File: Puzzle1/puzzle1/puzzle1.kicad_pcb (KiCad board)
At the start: 2 copper layers, 125 x 100 mm, 28 parts, among them J1 Conn_01x04_Pin, J10 Conn_01x09_Socket, J11 Conn_01x04_Socket, J12 Conn_01x04_Socket, J13 Conn_01x04_Socket, J14 Conn_01x04_Socket, J2 Conn_01x09_Socket, J3 Conn_01x09_Socket, J4 Conn_01x09_Socket, J5 Conn_01x09_Socket, J6 Conn_01x09_Socket, J7 Conn_01x09_Socket, J8 Conn_01x09_Socket, J9 Conn_01x09_Socket, U1 PCA9555D, U2 PCA9555D, U3 PCA9555D, U4 PCA9555D, U5 PCA9555D, U6 PCA9555D

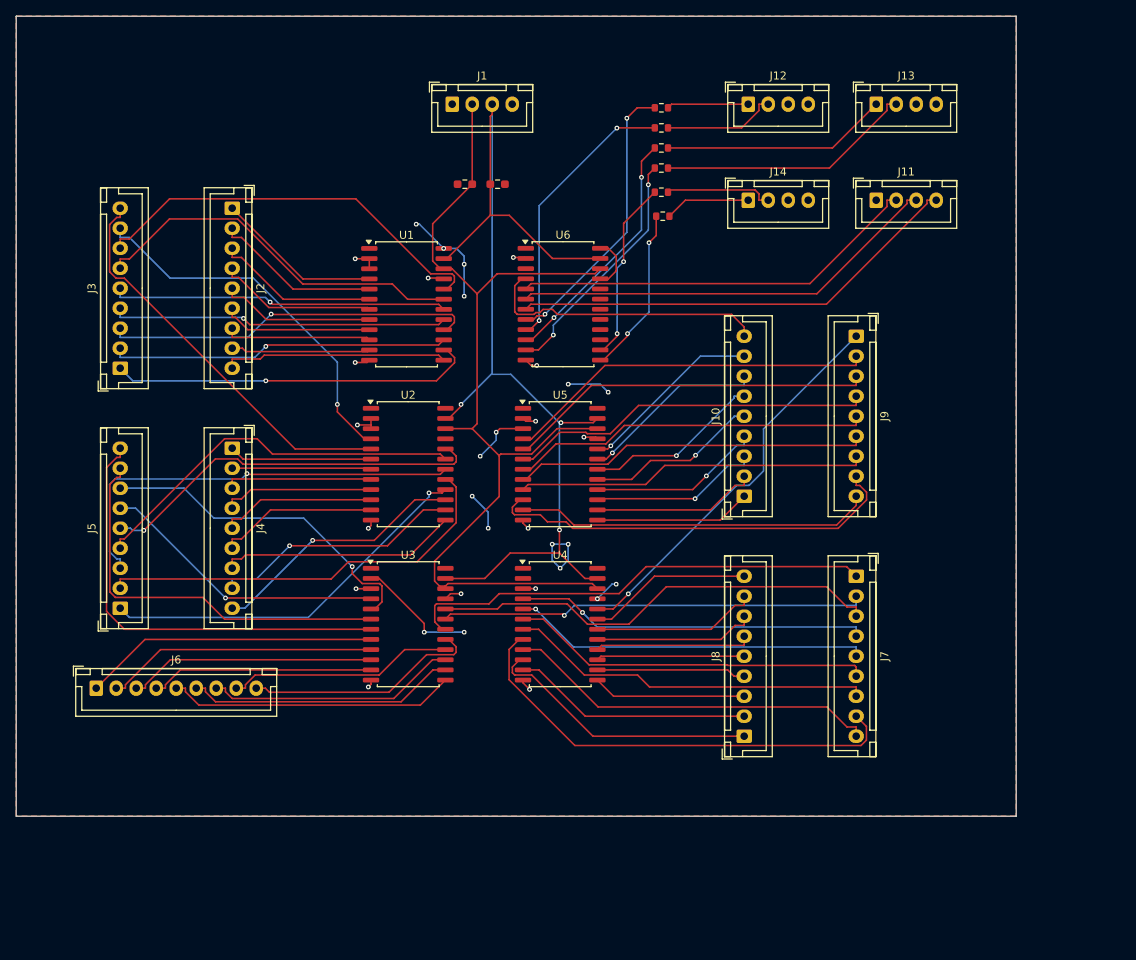
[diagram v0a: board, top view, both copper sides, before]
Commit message: update after review
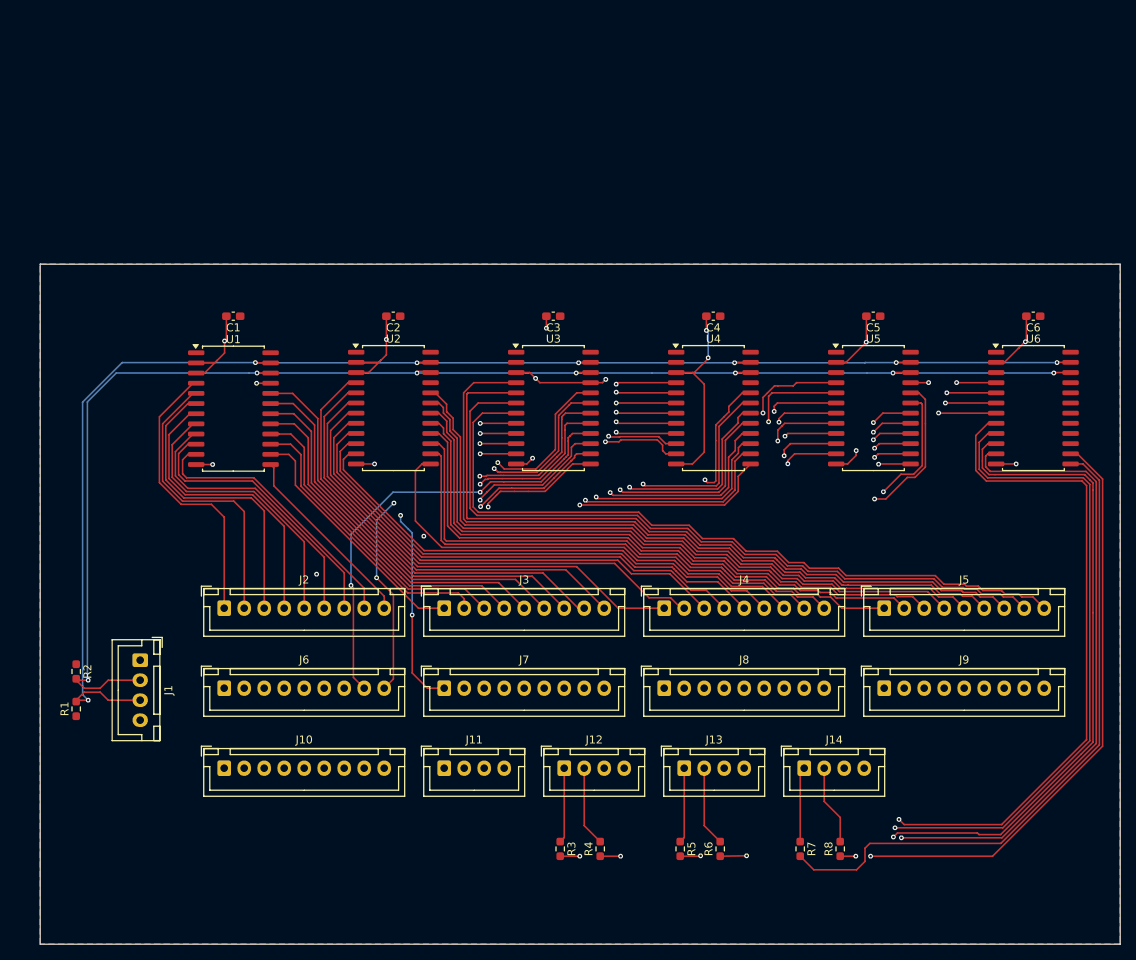
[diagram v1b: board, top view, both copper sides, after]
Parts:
- added C1: 100n, Capacitor_SMD:C_0603_1608Metric_Pad1.08x0.95mm_HandSolder, F.Cu at (49.1, 56.5)
- added C2: 100n, Capacitor_SMD:C_0603_1608Metric_Pad1.08x0.95mm_HandSolder, F.Cu at (69.1, 56.5)
- added C3: 100n, Capacitor_SMD:C_0603_1608Metric_Pad1.08x0.95mm_HandSolder, F.Cu at (89.1, 56.5)
- added C4: 100n, Capacitor_SMD:C_0603_1608Metric_Pad1.08x0.95mm_HandSolder, F.Cu at (109.1, 56.5)
- added C5: 100n, Capacitor_SMD:C_0603_1608Metric_Pad1.08x0.95mm_HandSolder, F.Cu at (129.1, 56.5)
- added C6: 100n, Capacitor_SMD:C_0603_1608Metric_Pad1.08x0.95mm_HandSolder, F.Cu at (149.1, 56.5)
- J10, J2, J3, J4, J5, J6, J7, J8, J9: value Conn_01x09_Socket -> Conn_01x09_Pin
- J11, J12, J13, J14: value Conn_01x04_Socket -> Conn_01x04_Pin
- R3, R4, R5, R6, R7, R8: footprint Resistor_SMD:R_0603_1608Metric -> Resistor_SMD:R_0603_1608Metric_Pad0.98x0.95mm_HandSolder
- moved J5 95.5 mm to (130.5, 93.0), turned to 0 degrees
- moved R3 93.5 mm to (90.0, 123.1), turned to -90 degrees
- moved R4 90.5 mm to (95.0, 123.1), turned to 90 degrees
- moved J11 89.2 mm to (75.5, 113.0)
- moved R5 87.6 mm to (105.0, 123.1), turned to -90 degrees
- moved J13 86.4 mm to (105.5, 113.0)
- moved J12 86.1 mm to (90.5, 113.0)
- moved R6 85.4 mm to (110.0, 123.1), turned to 90 degrees
- moved R8 85.1 mm to (125.0, 123.1), turned to 90 degrees
- moved R1 84.1 mm to (29.5, 105.6), turned to 90 degrees
- moved R7 80.9 mm to (120.0, 123.1), turned to -90 degrees
- moved J1 79.7 mm to (37.5, 99.5), turned to -90 degrees
- moved R2 77.9 mm to (29.5, 100.9), turned to -90 degrees
- moved J10 73.4 mm to (48.0, 113.0), turned to 0 degrees
- moved J14 71.3 mm to (120.5, 113.0)
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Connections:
- net +5V renamed VCC
- net 1 renamed /Connectors/GPIO_64
- net 6 renamed /Connectors/GPIO_33
- net 7 renamed /Connectors/GPIO_34
- net 8 renamed /Connectors/GPIO_35
- net 9 renamed /Connectors/GPIO_36
- net Net-(J10-Pin_1) renamed /Connectors/GPIO_73
- net Net-(J10-Pin_2) renamed /Connectors/GPIO_74
- net Net-(J10-Pin_3) renamed /Connectors/GPIO_75
- net Net-(J10-Pin_4) renamed /Connectors/GPIO_76
- net Net-(J10-Pin_5) renamed /Connectors/GPIO_77
- net Net-(J10-Pin_6) renamed /Connectors/GPIO_78
- net Net-(J10-Pin_7) renamed /Connectors/GPIO_79
- net Net-(J10-Pin_8) renamed /Connectors/GPIO_80
- net Net-(J10-Pin_9) renamed /Connectors/GPIO_81
- net Net-(J11-Pin_2) renamed /Connectors/GPIO_82
- net Net-(J11-Pin_3) renamed /Connectors/GPIO_83
- net Net-(J11-Pin_4) renamed /Connectors/GPIO_84
- net Net-(J2-Pin_1) renamed /Connectors/GPIO_1
- net Net-(J2-Pin_2) renamed /Connectors/GPIO_2
- net Net-(J2-Pin_3) renamed /Connectors/GPIO_3
- net Net-(J2-Pin_4) renamed /Connectors/GPIO_4
- net Net-(J2-Pin_5) renamed /Connectors/GPIO_5
- net Net-(J2-Pin_6) renamed /Connectors/GPIO_6
- net Net-(J2-Pin_7) renamed /Connectors/GPIO_7
- net Net-(J2-Pin_8) renamed /Connectors/GPIO_8
- net Net-(J2-Pin_9) renamed /Connectors/GPIO_9
- net Net-(J3-Pin_1) renamed /Connectors/GPIO_10
- net Net-(J3-Pin_2) renamed /Connectors/GPIO_11
- net Net-(J3-Pin_3) renamed /Connectors/GPIO_12
- net Net-(J3-Pin_4) renamed /Connectors/GPIO_13
- net Net-(J3-Pin_5) renamed /Connectors/GPIO_14
- net Net-(J3-Pin_6) renamed /Connectors/GPIO_15
- net Net-(J3-Pin_7) renamed /Connectors/GPIO_16
- net Net-(J3-Pin_8) renamed /Connectors/GPIO_17
- net Net-(J3-Pin_9) renamed /Connectors/GPIO_18
- net Net-(J4-Pin_1) renamed /Connectors/GPIO_19
- net Net-(J4-Pin_2) renamed /Connectors/GPIO_20
- net Net-(J4-Pin_3) renamed /Connectors/GPIO_21
- net Net-(J4-Pin_4) renamed /Connectors/GPIO_22
- net Net-(J4-Pin_5) renamed /Connectors/GPIO_23
- net Net-(J4-Pin_6) renamed /Connectors/GPIO_24
- net Net-(J4-Pin_7) renamed /Connectors/GPIO_25
- net Net-(J4-Pin_8) renamed /Connectors/GPIO_26
- net Net-(J4-Pin_9) renamed /Connectors/GPIO_27
- net Net-(J5-Pin_1) renamed /Connectors/GPIO_28
- net Net-(J5-Pin_2) renamed /Connectors/GPIO_29
- net Net-(J5-Pin_3) renamed /Connectors/GPIO_30
- net Net-(J5-Pin_4) renamed /Connectors/GPIO_31
- net Net-(J5-Pin_5) renamed /Connectors/GPIO_32
- net Net-(J6-Pin_1) renamed /Connectors/GPIO_37
- net Net-(J6-Pin_2) renamed /Connectors/GPIO_38
- net Net-(J6-Pin_3) renamed /Connectors/GPIO_39
- net Net-(J6-Pin_4) renamed /Connectors/GPIO_40
- net Net-(J6-Pin_5) renamed /Connectors/GPIO_41
- net Net-(J6-Pin_6) renamed /Connectors/GPIO_42
- net Net-(J6-Pin_7) renamed /Connectors/GPIO_43
- net Net-(J6-Pin_8) renamed /Connectors/GPIO_44
- net Net-(J6-Pin_9) renamed /Connectors/GPIO_45
- net Net-(J7-Pin_1) renamed /Connectors/GPIO_46
- net Net-(J7-Pin_2) renamed /Connectors/GPIO_47
- net Net-(J7-Pin_3) renamed /Connectors/GPIO_48
- net Net-(J7-Pin_4) renamed /Connectors/GPIO_49
- net Net-(J7-Pin_5) renamed /Connectors/GPIO_50
- net Net-(J7-Pin_6) renamed /Connectors/GPIO_51
- net Net-(J7-Pin_7) renamed /Connectors/GPIO_52
- net Net-(J7-Pin_8) renamed /Connectors/GPIO_53
- net Net-(J7-Pin_9) renamed /Connectors/GPIO_54
- net Net-(J8-Pin_1) renamed /Connectors/GPIO_55
- net Net-(J8-Pin_2) renamed /Connectors/GPIO_56
- net Net-(J8-Pin_3) renamed /Connectors/GPIO_57
- net Net-(J8-Pin_4) renamed /Connectors/GPIO_58
- net Net-(J8-Pin_5) renamed /Connectors/GPIO_59
- net Net-(J8-Pin_6) renamed /Connectors/GPIO_60
- net Net-(J8-Pin_7) renamed /Connectors/GPIO_61
- net Net-(J8-Pin_8) renamed /Connectors/GPIO_62
- net Net-(J8-Pin_9) renamed /Connectors/GPIO_63
- net Net-(J9-Pin_2) renamed /Connectors/GPIO_65
- net Net-(J9-Pin_3) renamed /Connectors/GPIO_66
- net Net-(J9-Pin_4) renamed /Connectors/GPIO_67
- net Net-(J9-Pin_5) renamed /Connectors/GPIO_68
- net Net-(J9-Pin_6) renamed /Connectors/GPIO_69
- net Net-(J9-Pin_7) renamed /Connectors/GPIO_70
- net Net-(J9-Pin_8) renamed /Connectors/GPIO_71
- net Net-(J9-Pin_9) renamed /Connectors/GPIO_72
- net Net-(U6-IO0_4) renamed /Connectors/GPIO_85
- net Net-(U6-IO0_6) renamed /Connectors/GPIO_87
- net Net-(U6-IO1_0) renamed /Connectors/GPIO_89
- net SCL renamed /SCL
- net SDA renamed /SDA
- R4 pad 1: Net-(J12-Pin_2) -> /Connectors/GPIO_86
- R4 pad 2: Net-(U6-IO0_5) -> Net-(J12-Pin_2)
- R6 pad 1: Net-(J13-Pin_2) -> /Connectors/GPIO_88
- R6 pad 2: Net-(U6-IO0_7) -> Net-(J13-Pin_2)
- R8 pad 1: Net-(J14-Pin_2) -> /Connectors/GPIO_90
- R8 pad 2: Net-(U6-IO1_1) -> Net-(J14-Pin_2)
- U6 pad 11: Net-(U6-IO0_7) -> /Connectors/GPIO_88
- U6 pad 14: Net-(U6-IO1_1) -> /Connectors/GPIO_90
- U6 pad 15: unconnected-(U6-IO1_2-Pad15) -> /Connectors/GPIO_91
- U6 pad 16: unconnected-(U6-IO1_3-Pad16) -> /Connectors/GPIO_92
- U6 pad 17: unconnected-(U6-IO1_4-Pad17) -> /Connectors/GPIO_93
- U6 pad 18: unconnected-(U6-IO1_5-Pad18) -> /Connectors/GPIO_94
- U6 pad 19: unconnected-(U6-IO1_6-Pad19) -> /Connectors/GPIO_95
- U6 pad 20: unconnected-(U6-IO1_7-Pad20) -> /Connectors/GPIO_96
- U6 pad 9: Net-(U6-IO0_5) -> /Connectors/GPIO_86
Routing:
- net /Connectors/GPIO_86: track 0.00 -> 119.8 mm, vias 0 -> 2
- net /Connectors/GPIO_88: track 0.00 -> 103.1 mm, vias 0 -> 2
- net /Connectors/GPIO_85: track 35.4 -> 126.4 mm
- net /Connectors/GPIO_74: track 20.8 -> 110.8 mm, vias 0 -> 1
- net /Connectors/GPIO_73: track 19.6 -> 109.4 mm, vias 0 -> 1
- net /Connectors/GPIO_75: track 21.3 -> 110.6 mm
- net /Connectors/GPIO_76: track 21.8 -> 109.9 mm
- net /Connectors/GPIO_77: track 21.7 -> 109.1 mm
- net /Connectors/GPIO_78: track 22.3 -> 109.7 mm
- net /Connectors/GPIO_80: track 23.2 -> 106.3 mm
- net /Connectors/GPIO_79: track 23.3 -> 105.9 mm
- net /Connectors/GPIO_87: track 31.1 -> 109.1 mm
- net /Connectors/GPIO_90: track 0.00 -> 77.2 mm, vias 0 -> 2
- net /Connectors/GPIO_81: track 36.1 -> 112.3 mm, vias 0 -> 1
- net GND: track 27.3 -> 96.7 mm, vias 15 -> 16
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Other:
- board size 125 x 100 mm -> 135 x 85 mm
- copper layers 2 -> 4
